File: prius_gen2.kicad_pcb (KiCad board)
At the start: 4 copper layers, 147.8 x 65 mm, 138 parts, among them J1 Conn_02x05_Odd_Even, J2 Conn_01x06, J3 Conn_01x23, J4 Conn_01x14, Q1 Q_NPN_BEC, Q2 Q_PNP_BEC, Q3 Q_NPN_BEC, Q4 Q_PNP_BEC, SW1 SW_Push, SW2 SW_Push, U1 STM32F407VETx, U2 ULN2003A, U3 AD2S1205YSTZ, U4 TJA1051T-3, U5 LMR14020, U6 AZ1117-3.3, U7 MCP602, U8 AD8676xR, Y1 8MHz, Y2 8.192MHz

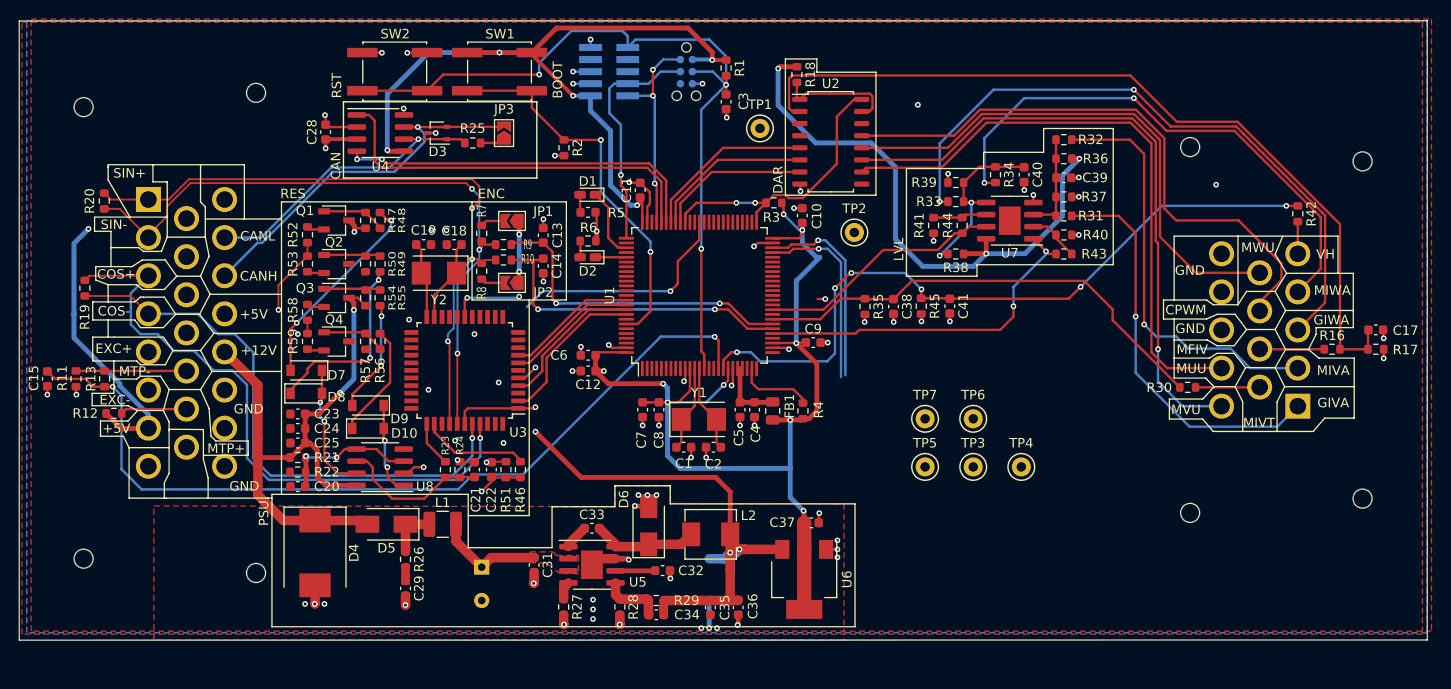
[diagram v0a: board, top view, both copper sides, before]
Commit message: cleaned up board
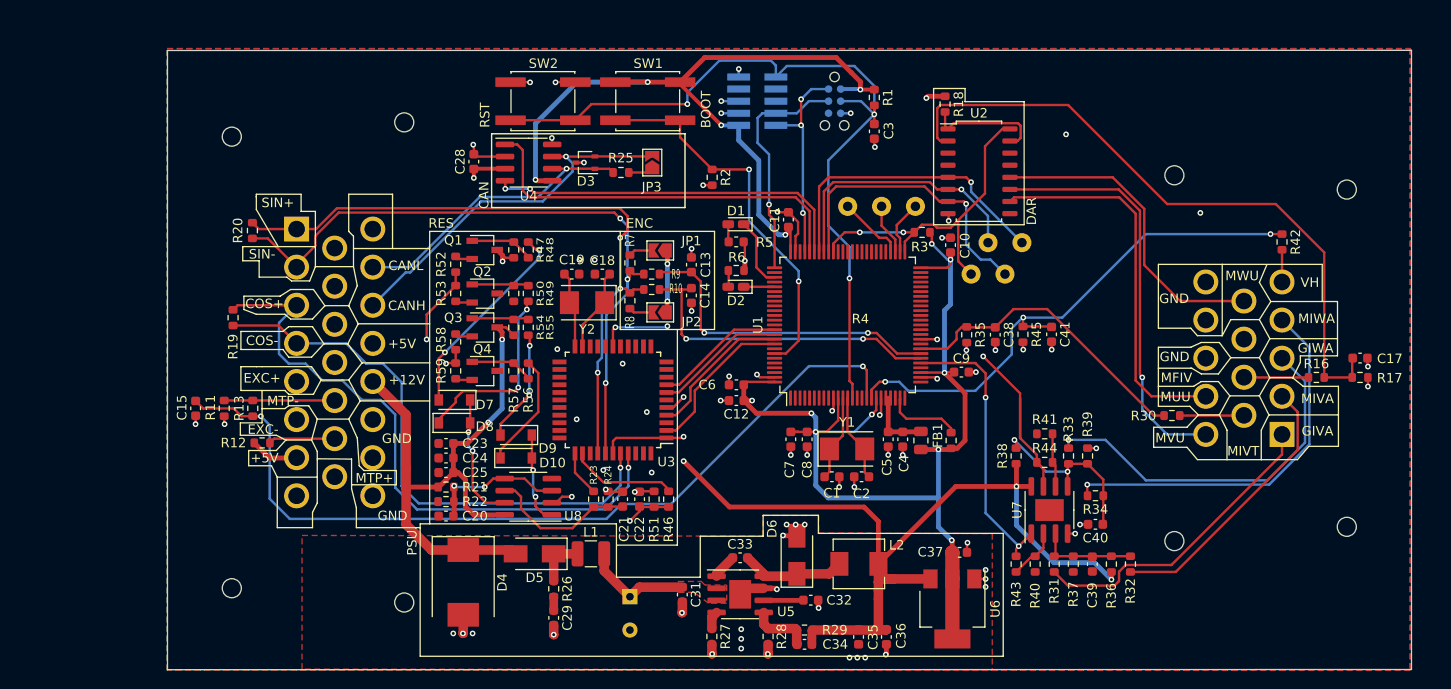
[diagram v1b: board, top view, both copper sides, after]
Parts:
- TP1, TP2, TP3, TP4, TP5, TP6, TP7: moved to B.Cu
- moved R32 45.1 mm to (183.4, 121.4), turned to -90 degrees
- moved R36 42.8 mm to (181.4, 121.4), turned to 90 degrees
- moved C39 40.7 mm to (179.4, 121.4), turned to -90 degrees
- moved R37 38.6 mm to (177.4, 121.4), turned to -90 degrees
- moved C40 37.5 mm to (179.7, 117.2), turned to 180 degrees
- moved R31 36.6 mm to (175.4, 121.4), turned to -90 degrees
- moved R34 35.3 mm to (179.7, 114.2), turned to 180 degrees
- moved R40 34.7 mm to (173.4, 121.4), turned to -90 degrees
- moved R43 32.9 mm to (171.4, 121.4), turned to 90 degrees
- moved R39 31.9 mm to (178.9, 110.1), turned to 90 degrees
- moved U7 30.7 mm to (174.9, 115.7), turned to 90 degrees
- moved TP3 30.4 mm to (153.7, 83.9), turned to 180 degrees
- moved R33 29.2 mm to (176.9, 110.1), turned to 90 degrees
- moved R44 26.3 mm to (174.4, 110.7), turned to 180 degrees
- moved R41 24.8 mm to (174.4, 107.7), turned to 180 degrees
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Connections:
- C13 pad 1: /Input Filter/TIM3_CH2 -> /TIM3_CH2
- C14 pad 1: /Input Filter/TIM3_CH1 -> /TIM3_CH1
- C38 pad 1: /Level Shifting/ADC14 -> /ADC14
- C41 pad 1: /Level Shifting/ADC13 -> /ADC13
- R10 pad 1: /Input Filter/TIM3_CH1 -> /TIM3_CH1
- R11 pad 1: /Input Filter/MTEMP- -> /MTEMP-
- R12 pad 1: /Input Filter/MTEMP+ -> /MTEMP+
- R13 pad 1: /Input Filter/MTEMP- -> /MTEMP-
- R30 pad 1: /Level Shifting/ADC14 -> /ADC14
- R30 pad 2: /Level Shifting/MIVT -> /MIVT
- R31 pad 2: /Level Shifting/GIVA -> /Connectors/GIVA
- R32 pad 2: /Level Shifting/MIVA -> /Connectors/MIVA
- R33 pad 2: /Level Shifting/GIWA -> /Connectors/GIWA
- R34 pad 2: /Level Shifting/MIWA -> /Connectors/MIWA
- R35 pad 1: /Level Shifting/ADC14 -> /ADC14
- R42 pad 1: /Level Shifting/ADC13 -> /ADC13
- R42 pad 2: /Level Shifting/VH -> /VH
- R43 pad 2: /Level Shifting/ADC5 -> /ADC5
- R44 pad 2: /Level Shifting/ADC8 -> /ADC8
- R45 pad 1: /Level Shifting/ADC13 -> /ADC13
- R9 pad 1: /Input Filter/TIM3_CH2 -> /TIM3_CH2
- U3 pad 2: /Resolver/~{RD} -> /~{CS}
- U3 pad 4: /Resolver/~{SAMPLE} -> /~{SAMPLE}
- U3 pad 7: /Resolver/SO -> /MISO
- U3 pad 8: /Resolver/SCLK -> /SCLK
- U4 pad 1: /Communication/TXDCAN -> /CAN_TX
- U4 pad 4: /Communication/RXDCAN -> /CAN_RX
- U7 pad 1: /Level Shifting/ADC5 -> /ADC5
- U7 pad 7: /Level Shifting/ADC8 -> /ADC8
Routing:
- net /Level Shifting/ADC13: track 75.5 -> 0.00 mm, vias 6 -> 0
- net /Level Shifting/GIWA: track 68.4 -> 0.00 mm, vias 2 -> 0
- net +5V: track 309.4 -> 245.3 mm, vias 14 -> 11
- net unconnected-(J4-Pad8): track 62.1 -> 0.00 mm
- net /ADC13: track 0.00 -> 56.9 mm, vias 0 -> 3
- net /Level Shifting/ADC14: track 49.8 -> 0.00 mm
- net /Level Shifting/MIVA: track 44.1 -> 0.00 mm, vias 1 -> 0
- net /Level Shifting/GIVA: track 42.4 -> 0.00 mm, vias 1 -> 0
- net /Connectors/GIWA: track 0.00 -> 39.0 mm, vias 0 -> 1
- net /Communication/RXDCAN: track 38.6 -> 0.00 mm, vias 2 -> 0
- net /CAN_RX: track 0.00 -> 38.6 mm, vias 0 -> 2
- net /Level Shifting/ADC5: track 37.3 -> 0.00 mm, vias 2 -> 0
- net /TIM3_CH1: track 0.00 -> 34.3 mm, vias 0 -> 2
- net /Input Filter/TIM3_CH1: track 34.3 -> 0.00 mm, vias 2 -> 0
- net /Input Filter/TIM3_CH2: track 34.2 -> 0.00 mm, vias 2 -> 0
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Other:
- board size 147.8 x 65 mm -> 130.6 x 65 mm
- board text removed: "CPWM"
- board text removed: "LVL"
